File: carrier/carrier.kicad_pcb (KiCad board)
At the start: 2 copper layers, 43 parts, among them J1 Connector, J2 Connector, J3 WeAct_1, J4 WeAct_2, J5 Seansor_Header_A, J6 Seansor_Header_B, U1 TPS54302, U2 SN65HVD230, U3 ATECC608B-SSHDA

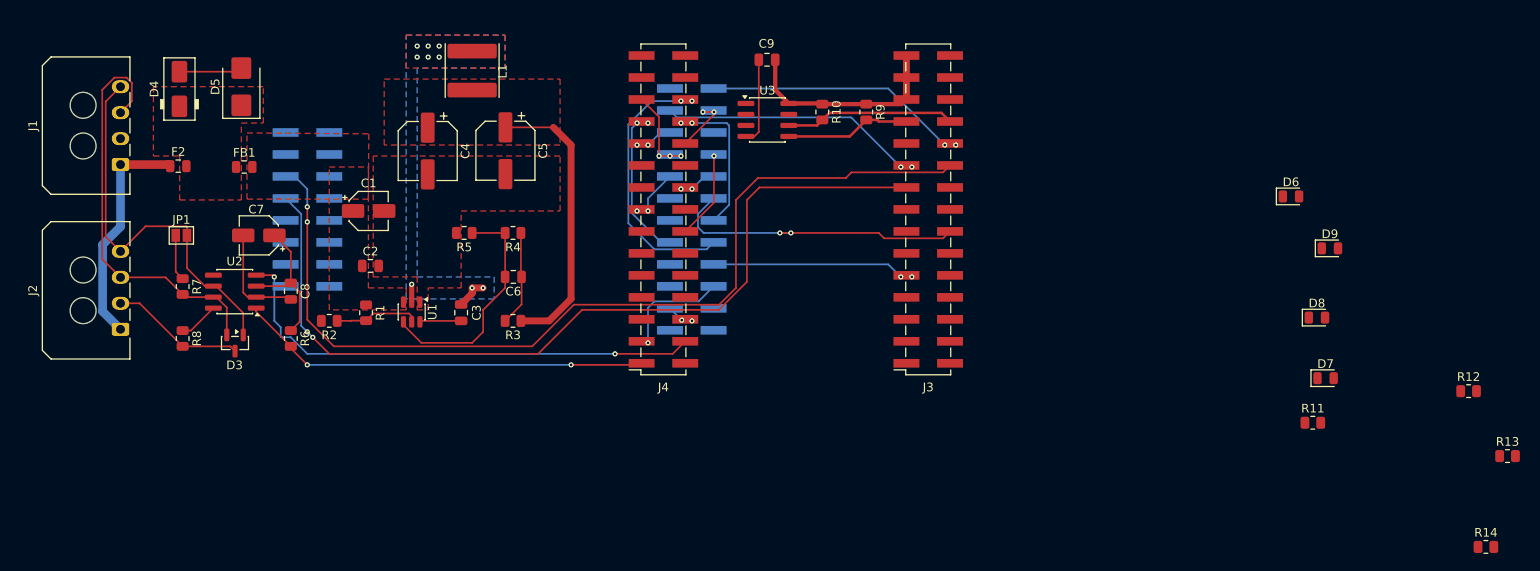
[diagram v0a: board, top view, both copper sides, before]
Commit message: Add files via upload
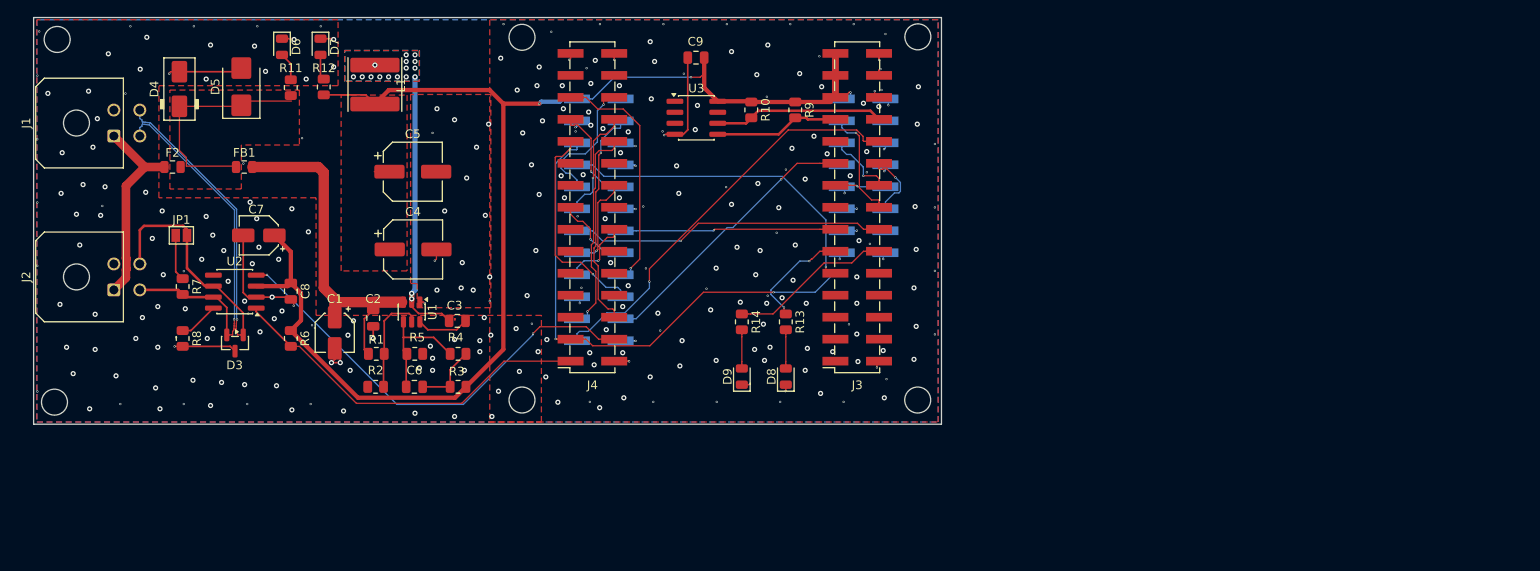
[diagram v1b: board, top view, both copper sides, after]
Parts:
- J1, J2: footprint Connector_Molex:Molex_Micro-Fit_3.0_43650-0400_1x04_P3.00mm_Horizontal -> Connector_Molex:Molex_Micro-Fit_3.0_43045-0400_2x02_P3.00mm_Horizontal
- moved R12 136.9 mm to (90.8, 28.9), turned to 90 degrees
- moved R11 124.3 mm to (87.0, 28.9), turned to 90 degrees
- moved D7 122.3 mm to (90.4, 24.2), turned to -90 degrees
- moved D6 117.9 mm to (86.0, 24.2), turned to -90 degrees
- moved R14 89.8 mm to (139.1, 56.0), turned to -90 degrees
- moved R13 84.8 mm to (144.2, 56.0), turned to -90 degrees
- moved D9 69.5 mm to (139.1, 62.3), turned to 90 degrees
- moved J6 64.4 mm to (153.2, 39.1), turned to 180 degrees
- moved D8 61.7 mm to (144.2, 62.3), turned to 90 degrees
- moved C6 17.1 mm to (101.3, 63.5)
- moved R4 15.3 mm to (106.3, 59.7)
- moved R5 15.1 mm to (101.3, 59.7), turned to 0 degrees
- moved C1 14.6 mm to (92.1, 57.3), turned to -90 degrees
- moved C4 11.5 mm to (101.1, 47.6), turned to 0 degrees
- moved L1 11.4 mm to (96.7, 28.6)
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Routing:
- net ADC_2: track 108.4 -> 7.88 mm, vias 2 -> 1
- net ADC_1: track 100.2 -> 5.85 mm, vias 2 -> 1
- net +3.3V: track 74.5 -> 152.3 mm, vias 0 -> 3
- net I2C1_SDA: track 12.7 -> 62.6 mm, vias 1 -> 2
- net Net-(U1-VIN): track 0.00 -> 39.4 mm
- net GND: track 46.2 -> 82.6 mm, vias 0 -> 292
- net Net-(U1-SW): track 5.77 -> 32.3 mm, vias 7 -> 17
- net +12V: track 0.17 -> 26.4 mm
- net SPI_CS2: track 0.00 -> 24.9 mm, vias 0 -> 1
- net I2C1_SCL: track 3.14 -> 27.0 mm, vias 2 -> 1
- net PWM_1: track 4.41 -> 24.3 mm, vias 2 -> 1
- net LED_Status: track 0.00 -> 18.9 mm
- net GPIO_4: track 9.90 -> 28.2 mm, vias 3 -> 1
- net PWM_2: track 6.28 -> 24.3 mm, vias 2 -> 1
- net PWM_4: track 30.7 -> 47.6 mm, vias 2 -> 1
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- added copper zone on B.Cu, net GND
- removed copper zone on F.Cu, net Net-(U1-VIN)
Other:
- board outline added: 104.9 x 47 mm
- copper layers 2 -> 4
